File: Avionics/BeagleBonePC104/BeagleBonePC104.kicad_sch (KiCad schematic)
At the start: 14 parts, among them U4 TJA1051T-3, U5 TMP36xS

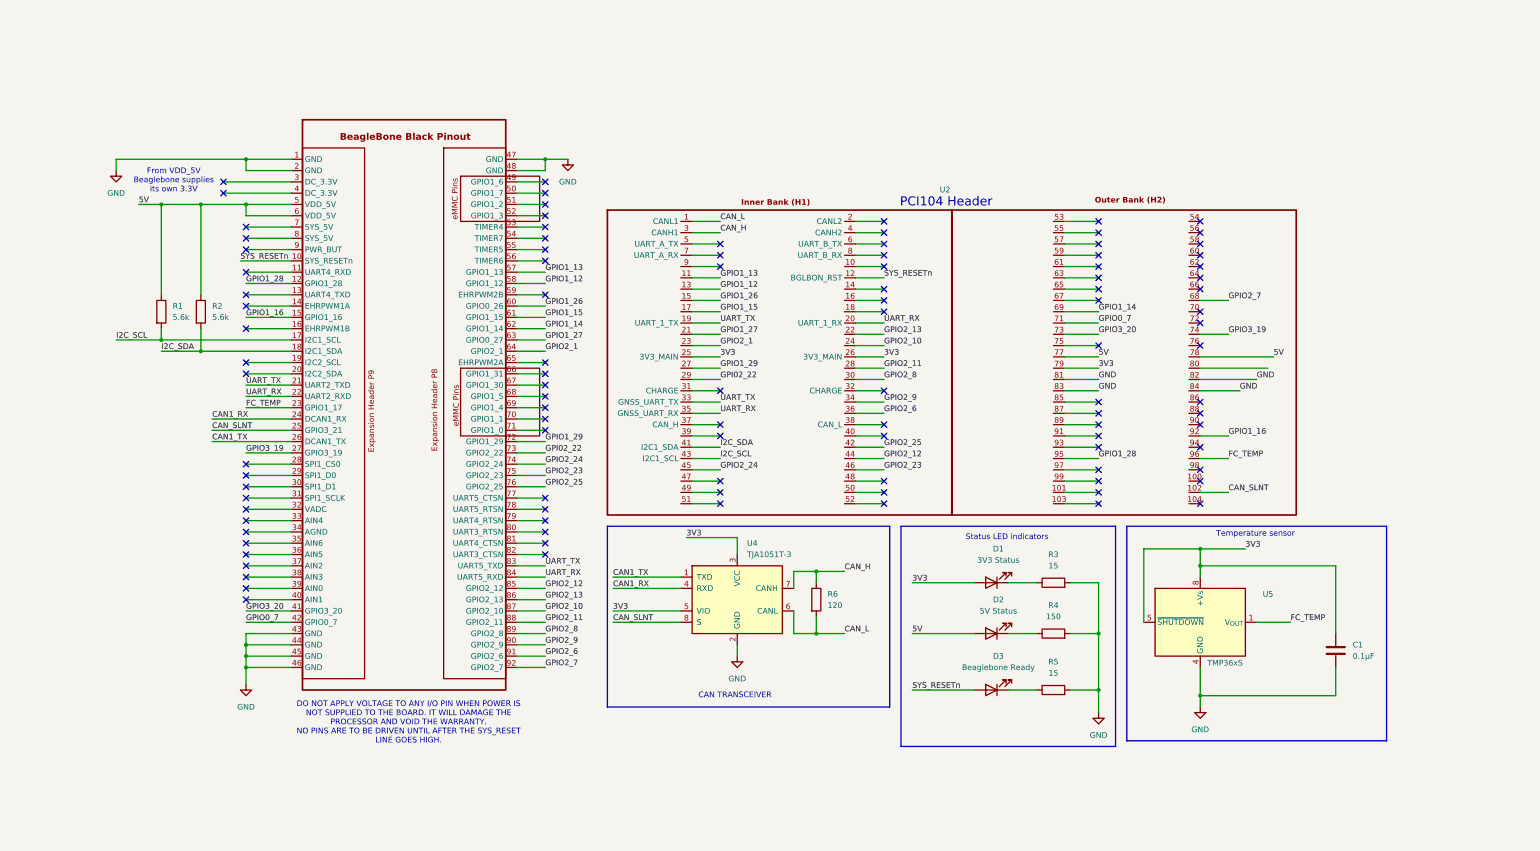
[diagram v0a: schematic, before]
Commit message: Ian Golberg - Tentatively Finalized v3 of the flight computer board.
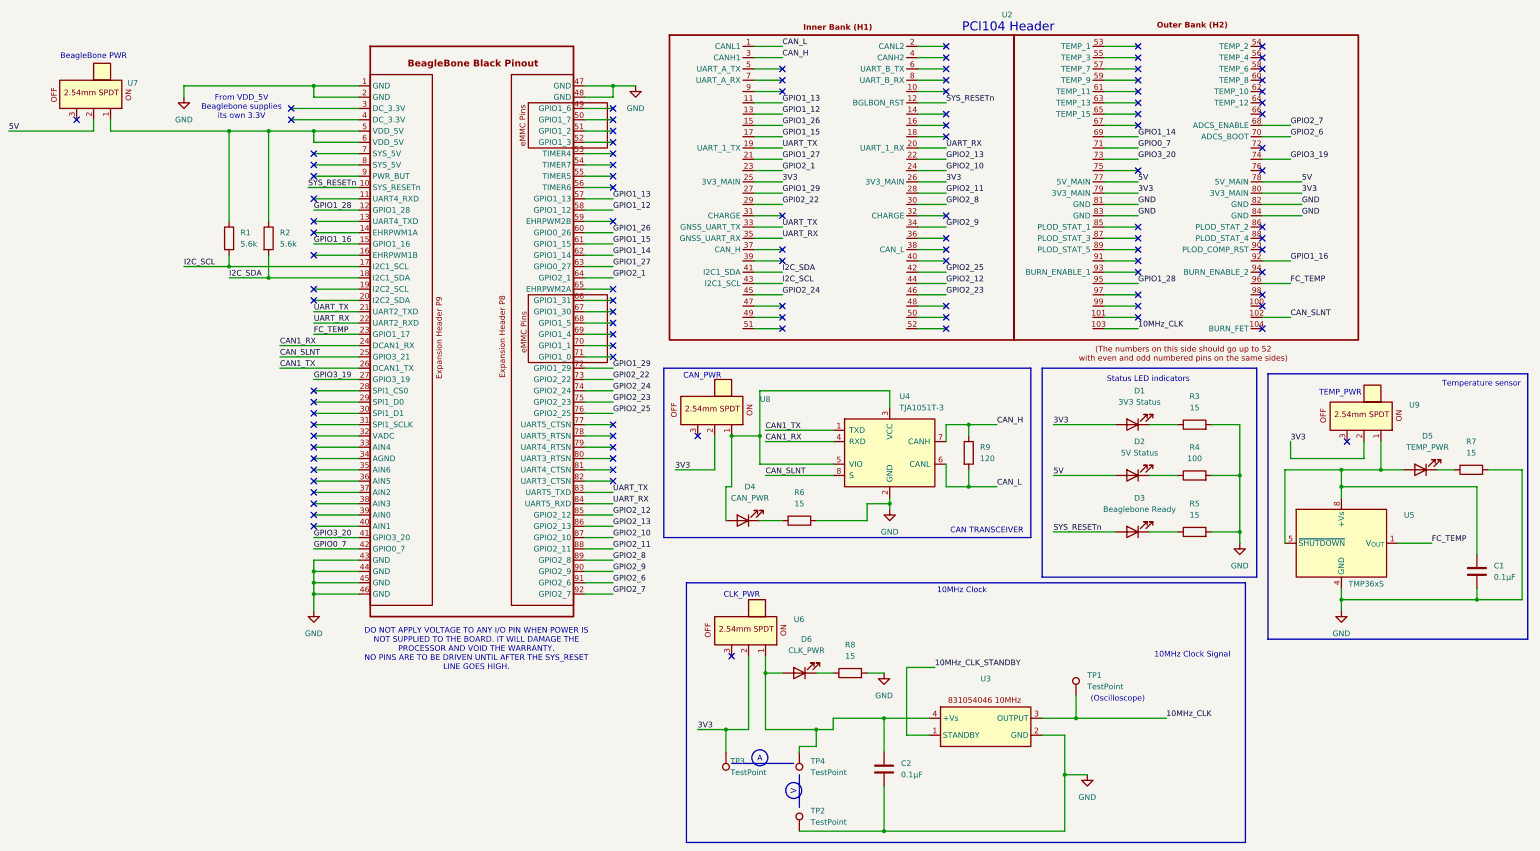
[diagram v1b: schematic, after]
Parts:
- added C2: 0.1µF, Capacitor_SMD:C_0805_2012Metric, symbol Device:C
- added D4: CAN_PWR, LED_SMD:LED_0805_2012Metric, symbol Device:LED
- added D5: TEMP_PWR, LED_SMD:LED_0805_2012Metric, symbol Device:LED
- added D6: CLK_PWR, LED_SMD:LED_0805_2012Metric, symbol Device:LED
- added R6, R7, R8: 15, Resistor_SMD:R_0805_2012Metric, symbol Device:R
- added TP1: TestPoint, TestPoint:TestPoint_Keystone_5000-5004_Miniature, symbol Connector:TestPoint
- added TP2, TP3, TP4: TestPoint, FlightCompuer:TestPointPad, symbol Connector:TestPoint
- added U3: ~, FlightCompuer:831054046, symbol FlightComputer:831054046_10MHz_Oscillator
- added U6, U7, U8, U9: ~, FlightCompuer:SPDT Through Hole Switch, symbol FlightComputer:2.54mm_Switch
- R4: value 150 -> 100; footprint Resistor_SMD:R_0603_1608Metric -> Resistor_SMD:R_0805_2012Metric
- U2: footprint PCI104Connector:PCI104ConnectorComplete -> PCI104Connector:PC104ConnectorFootprint
- renumbered R6 to R9
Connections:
- net 3V3: now also U2.80 (3V3_MAIN), TP3.1, U6.2, U8.2, U9.2; no longer C1.1, U4.3 (VCC), U4.5 (VIO), U5.5 (~{SHUTDOWN}), U5.8 (+Vs)
- net 5V: now also U7.2; no longer R1.1, R2.1, U1.5 (VDD_5V), U1.6 (VDD_5V)
- net GND: now also C2.2, R6.2, R7.2, R8.2, TP2.1, U3.2 (GND)
- net GPIO2_6: now also U2.70 (ADCS_BOOT); no longer U2.36
- net 10MHz_CLK: now reaches U2.103
- net 10MHz_CLK: now also TP1.1, U3.3 (OUTPUT)
- new net: R1.1, R2.1, U1.5 (VDD_5V), U1.6 (VDD_5V), U7.1
- new net: D6.1 (K), R8.1
- new net: C2.1, D6.2 (A), TP4.1, U3.4 (+Vs), U6.1
- new net: C1.1, D5.2 (A), U5.5 (~{SHUTDOWN}), U5.8 (+Vs), U9.1
- new net: D4.1 (K), R6.1
- new net: D4.2 (A), U4.3 (VCC), U4.5 (VIO), U8.1
- new net: D5.1 (K), R7.1
- new net 10MHz_CLK_STANDBY: U3.1 (STANDBY)
- no-connect marks 104 -> 107
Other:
- note added: "(Oscilloscope)"
- note added: "10MHz Clock"
- note added: "10MHz Clock Signal"
- note added: "A"
- note added: "BeagleBone PWR"
- note added: "CAN_PWR"
- note added: "CLK_PWR"
- note added: "TEMP_PWR"
- note added: "V"
- moved on the sheet: C1, D1, D2, D3, R1, R2, R3, R4, R5, R9, U4, U5
